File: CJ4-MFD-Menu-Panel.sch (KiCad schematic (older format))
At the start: 50 parts, among them SW1 SW_Push_LED, SW10 5_Way_Switch, SW11 SW_Push_LED, SW12 SW_Push_LED, SW13 SW_Push_LED, SW14 SW_Push_LED, SW15 SW_Push_LED, SW16 SW_Push_LED, SW17 SW_Push_LED, SW18 SW_Push_LED, SW19 SW_Push_LED, SW2 SW_Push_LED, SW20 SW_Push_LED, SW21 SW_Push_LED, SW3 SW_Push_LED, SW4 SW_Push_LED, SW5 SW_Push_LED, SW6 SW_Push_LED, SW7 SW_Push_LED, SW8 SW_Push_LED, SW9 SW_Push_LED, U1 MCP23017_SO, U2 MCP23017_SO, U3 IS31FL3733B

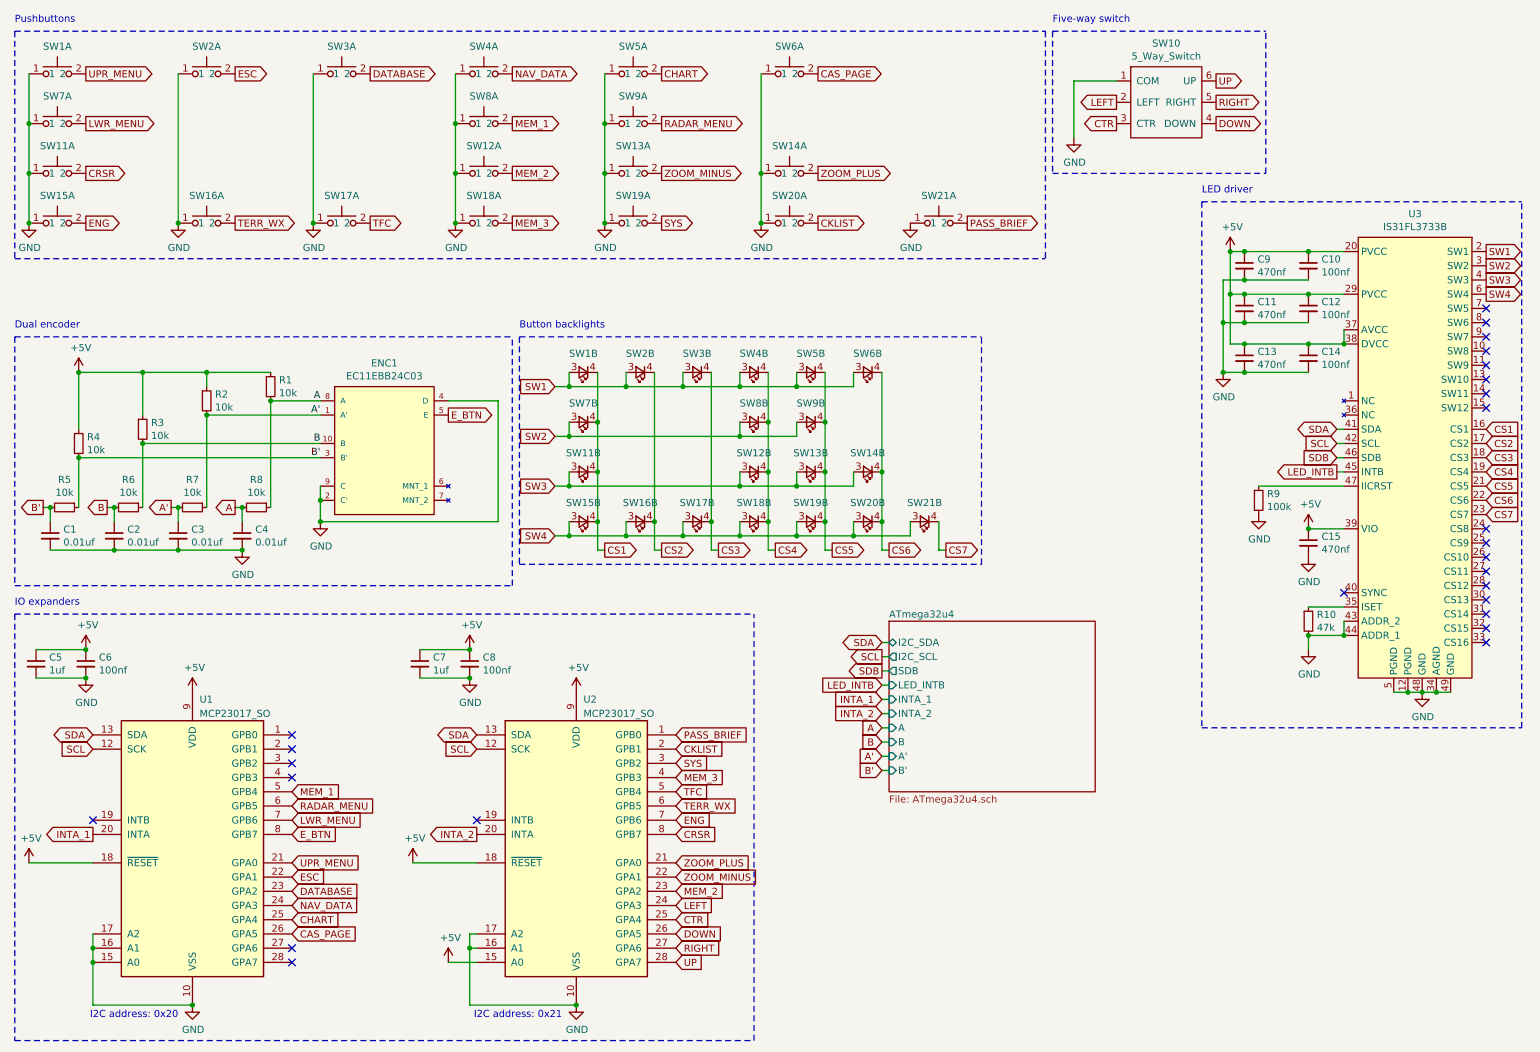
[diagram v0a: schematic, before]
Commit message: Fully routed and ready to go
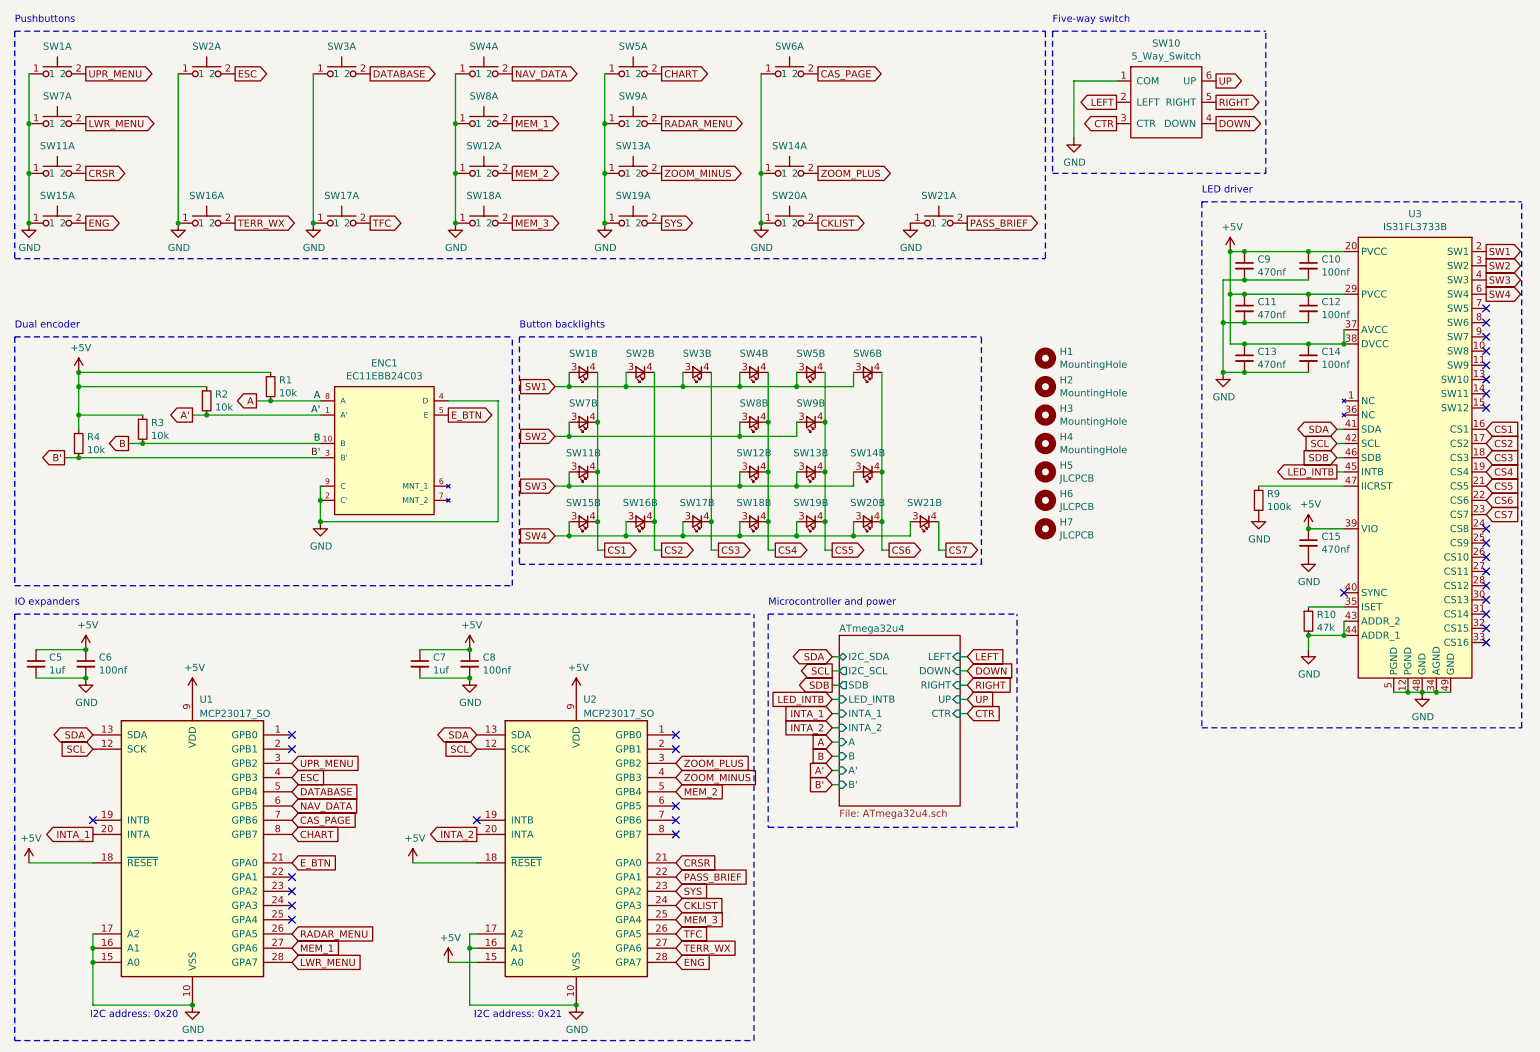
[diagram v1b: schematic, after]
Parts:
- removed C1, C2, C3, C4: 0.01uf, CJ4-MFD-Menu-Panel:Perfect_0402, symbol Device:C_Small
- removed R5, R6, R7, R8: 10k, CJ4-MFD-Menu-Panel:Perfect_0402, symbol Device:R_Small
- added H1, H2, H3, H4: MountingHole, MountingHole:MountingHole_3.2mm_M3, symbol Mechanical:MountingHole
- added H5, H6, H7: JLCPCB, CJ4-MFD-Menu-Panel:JLCPCB_Tooling_Hole, symbol Mechanical:MountingHole
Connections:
- net CAS_PAGE: now also U1.7 (GPB6); no longer U1.26 (GPA5)
- net CHART: now also U1.8 (GPB7); no longer U1.25 (GPA4)
- net CKLIST: now also U2.24 (GPA3); no longer U2.2 (GPB1)
- net CRSR: now also U2.21 (GPA0); no longer U2.8 (GPB7)
- net CTR: no longer U2.25 (GPA4)
- net DATABASE: now also U1.5 (GPB4); no longer U1.23 (GPA2)
- net DOWN: no longer U2.26 (GPA5)
- net ENG: now also U2.28 (GPA7); no longer U2.7 (GPB6)
- net ESC: now also U1.4 (GPB3); no longer U1.22 (GPA1)
- net E_BTN: now also U1.21 (GPA0); no longer U1.8 (GPB7)
- net LEFT: no longer U2.24 (GPA3)
- net LWR_MENU: now also U1.28 (GPA7); no longer U1.7 (GPB6)
- net MEM_1: now also U1.27 (GPA6); no longer U1.5 (GPB4)
- net MEM_2: now also U2.5 (GPB4); no longer U2.23 (GPA2)
- net MEM_3: now also U2.25 (GPA4); no longer U2.4 (GPB3)
- net NAV_DATA: now also U1.6 (GPB5); no longer U1.24 (GPA3)
- net PASS_BRIEF: now also U2.22 (GPA1); no longer U2.1 (GPB0)
- net RADAR_MENU: now also U1.26 (GPA5); no longer U1.6 (GPB5)
- net RIGHT: no longer U2.27 (GPA6)
- net SYS: now also U2.23 (GPA2); no longer U2.3 (GPB2)
- net TERR_WX: now also U2.27 (GPA6); no longer U2.6 (GPB5)
- net TFC: now also U2.26 (GPA5); no longer U2.5 (GPB4)
- net UP: no longer U2.28 (GPA7)
- net UPR_MENU: now also U1.3 (GPB2); no longer U1.21 (GPA0)
- net ZOOM_MINUS: now also U2.4 (GPB3); no longer U2.22 (GPA1)
- net ZOOM_PLUS: now also U2.3 (GPB2); no longer U2.21 (GPA0)
- no-connect marks 26 -> 31
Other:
- note added: "Microcontroller and power"

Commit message: Miscellaneous fixes
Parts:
- C10, C11, C12, C13, C14, C15, C5, C6, C7, C8, C9: JLC (none) -> 0402
- R1, R2, R3, R4: JLC (none) -> 0402; LCSC (none) -> C25744
- R10: JLC (none) -> 0402; LCSC (none) -> C25792
- R9: JLC (none) -> 0402; LCSC (none) -> C25741
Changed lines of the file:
@@
 F 2 "CJ4-MFD-Menu-Panel:Perfect_0402" H 1000 3550 50  0001 C CNN
 F 3 "~" H 1000 3550 50  0001 C CNN
+F 4 "0402" H 1000 3550 50  0001 C CNN "JLC"
+F 5 "C25744" H 1000 3550 50  0001 C CNN "LCSC"
 	1    1000 3550
 	1    0    0    -1
@@
 F 2 "CJ4-MFD-Menu-Panel:Perfect_0402" H 1450 3450 50  0001 C CNN
 F 3 "~" H 1450 3450 50  0001 C CNN
+F 4 "0402" H 1450 3450 50  0001 C CNN "JLC"
+F 5 "C25744" H 1450 3450 50  0001 C CNN "LCSC"
 	1    1450 3450
 	1    0    0    -1
@@
 F 2 "CJ4-MFD-Menu-Panel:Perfect_0402" H 1050 5100 50  0001 C CNN
 F 3 "~" H 1050 5100 50  0001 C CNN
+F 4 "0402" H 1050 5100 50  0001 C CNN "JLC"
 	1    1050 5100
 	1    0    0    -1
@@
 F 2 "CJ4-MFD-Menu-Panel:Perfect_0402" H 700 5100 50  0001 C CNN
 F 3 "~" H 700 5100 50  0001 C CNN
+F 4 "0402" H 700 5100 50  0001 C CNN "JLC"
 	1    700  5100
 	1    0    0    -1
@@
 F 2 "CJ4-MFD-Menu-Panel:Perfect_0402" H 3750 5100 50  0001 C CNN
 F 3 "~" H 3750 5100 50  0001 C CNN
+F 4 "0402" H 3750 5100 50  0001 C CNN "JLC"
 	1    3750 5100
 	1    0    0    -1
@@
 F 2 "CJ4-MFD-Menu-Panel:Perfect_0402" H 3400 5100 50  0001 C CNN
 F 3 "~" H 3400 5100 50  0001 C CNN
+F 4 "0402" H 3400 5100 50  0001 C CNN "JLC"
 	1    3400 5100
 	1    0    0    -1
@@
 F 2 "CJ4-MFD-Menu-Panel:Perfect_0402" H 9650 4800 50  0001 C CNN
 F 3 "~" H 9650 4800 50  0001 C CNN
+F 4 "0402" H 9650 4800 50  0001 C CNN "JLC"
+F 5 "C25792" H 9650 4800 50  0001 C CNN "LCSC"
 	1    9650 4800
 	1    0    0    -1
@@
 F 2 "CJ4-MFD-Menu-Panel:Perfect_0402" H 9650 4250 50  0001 C CNN
 F 3 "~" H 9650 4250 50  0001 C CNN
+F 4 "0402" H 9650 4250 50  0001 C CNN "JLC"
 	1    9650 4250
 	1    0    0    -1
@@
 F 2 "CJ4-MFD-Menu-Panel:Perfect_0402" H 9300 3950 50  0001 C CNN
 F 3 "~" H 9300 3950 50  0001 C CNN
+F 4 "0402" H 9300 3950 50  0001 C CNN "JLC"
+F 5 "C25741" H 9300 3950 50  0001 C CNN "LCSC"
 	1    9300 3950
 	1    0    0    -1
@@
 F 2 "CJ4-MFD-Menu-Panel:Perfect_0402" H 9650 2300 50  0001 C CNN
 F 3 "~" H 9650 2300 50  0001 C CNN
+F 4 "0402" H 9650 2300 50  0001 C CNN "JLC"
 	1    9650 2300
 	1    0    0    -1
@@
 F 2 "CJ4-MFD-Menu-Panel:Perfect_0402" H 9200 2300 50  0001 C CNN
 F 3 "~" H 9200 2300 50  0001 C CNN
+F 4 "0402" H 9200 2300 50  0001 C CNN "JLC"
 	1    9200 2300
 	1    0    0    -1
@@
 F 2 "CJ4-MFD-Menu-Panel:Perfect_0402" H 9650 2600 50  0001 C CNN
 F 3 "~" H 9650 2600 50  0001 C CNN
+F 4 "0402" H 9650 2600 50  0001 C CNN "JLC"
 	1    9650 2600
 	1    0    0    -1
@@
 F 2 "CJ4-MFD-Menu-Panel:Perfect_0402" H 9200 2600 50  0001 C CNN
 F 3 "~" H 9200 2600 50  0001 C CNN
+F 4 "0402" H 9200 2600 50  0001 C CNN "JLC"
 	1    9200 2600
 	1    0    0    -1
@@
 F 2 "CJ4-MFD-Menu-Panel:Perfect_0402" H 9650 2950 50  0001 C CNN
 F 3 "~" H 9650 2950 50  0001 C CNN
+F 4 "0402" H 9650 2950 50  0001 C CNN "JLC"
 	1    9650 2950
 	1    0    0    -1
@@
 F 2 "CJ4-MFD-Menu-Panel:Perfect_0402" H 9200 2950 50  0001 C CNN
 F 3 "~" H 9200 2950 50  0001 C CNN
+F 4 "0402" H 9200 2950 50  0001 C CNN "JLC"
 	1    9200 2950
 	1    0    0    -1
@@
 F 2 "CJ4-MFD-Menu-Panel:Perfect_0402" H 1900 3250 50  0001 C CNN
 F 3 "~" H 1900 3250 50  0001 C CNN
+F 4 "0402" H 1900 3250 50  0001 C CNN "JLC"
+F 5 "C25744" H 1900 3250 50  0001 C CNN "LCSC"
 	1    1900 3250
 	1    0    0    -1
@@
 F 2 "CJ4-MFD-Menu-Panel:Perfect_0402" H 2350 3150 50  0001 C CNN
 F 3 "~" H 2350 3150 50  0001 C CNN
+F 4 "0402" H 2350 3150 50  0001 C CNN "JLC"
+F 5 "C25744" H 2350 3150 50  0001 C CNN "LCSC"
 	1    2350 3150
 	1    0    0    -1
